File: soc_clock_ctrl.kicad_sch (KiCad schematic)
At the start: 15 parts, among them J4 Conn_01x03, J5 Conn_01x03, U4 MCIMX6Y2DVM09AB, Y1 24MHz, Y2 32.768kHz

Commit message: Update fields
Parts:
- C92, C93, C94, C95: Manufacturer (none) -> YAGEO; MfgPartNo (none) -> CC0402JRNPO9BN180; Vendor (none) -> Digi-Key; VendorPartNo (none) -> 311-1415-1-ND
- J4, J5: Manufacturer (none) -> Sullins Connector; MfgPartNo (none) -> GRPB031VWTC-RC; Vendor (none) -> Digi-Key; VendorPartNo (none) -> S9011E-03-ND
- JP1, TP6, TP7: Manufacturer (none) -> N/A; MfgPartNo (none) -> N/A; Vendor (none) -> N/A; VendorPartNo (none) -> N/A
- R44: Manufacturer (none) -> KOA Speer; MfgPartNo (none) -> RK73H1ETTP2204F; Vendor (none) -> Digi-Key; VendorPartNo (none) -> 2019-RK73H1ETTP2204FCT-ND
- R45: Manufacturer (none) -> YAGEO; MfgPartNo (none) -> RC0402FR-07100KL; Vendor (none) -> Digi-Key; VendorPartNo (none) -> 311-100KLRCT-ND
- R46: Manufacturer (none) -> YAGEO; MfgPartNo (none) -> RC0402JR-0710KL; Vendor (none) -> Digi-Key; VendorPartNo (none) -> 311-10KJRCT-ND
- Y1: Manufacturer (none) -> Raltron Electronics; MfgPartNo (none) -> H130B-24.000-18-2020-TR; Vendor (none) -> Digi-Key; VendorPartNo (none) -> 2151-H130B-24.000-18-2020-TRCT-ND
- Y2: Manufacturer (none) -> EPSON; MfgPartNo (none) -> FC-12M 32.7680KA-AC3; Vendor (none) -> Digi-Key; VendorPartNo (none) -> SER4081CT-ND

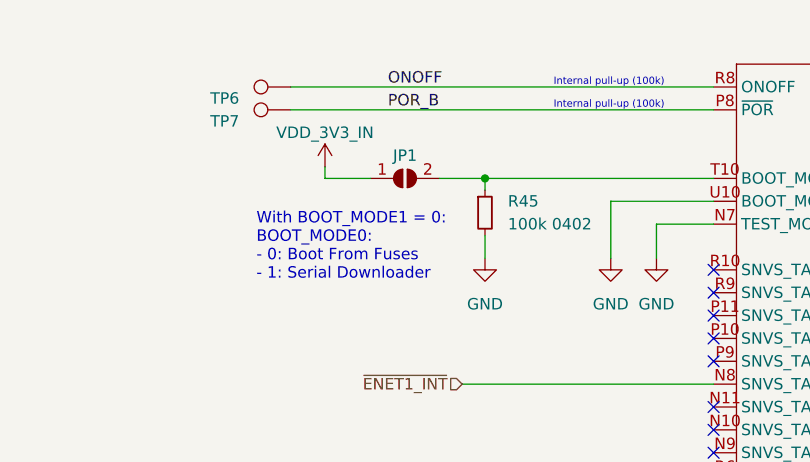
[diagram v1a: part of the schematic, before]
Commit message: KiCad 7
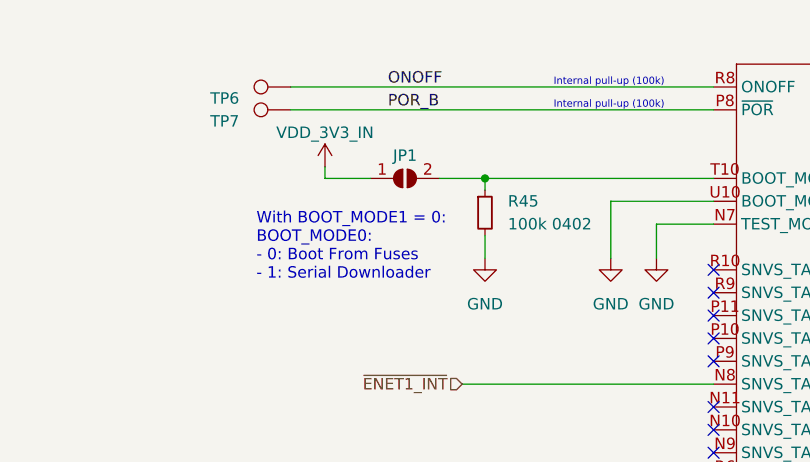
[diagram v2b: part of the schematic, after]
